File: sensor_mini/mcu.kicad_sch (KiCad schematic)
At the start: 13 parts, among them J2 Programming Header, U8 PIC18LF26K83, U9 MCP2562, Y1 Crystal

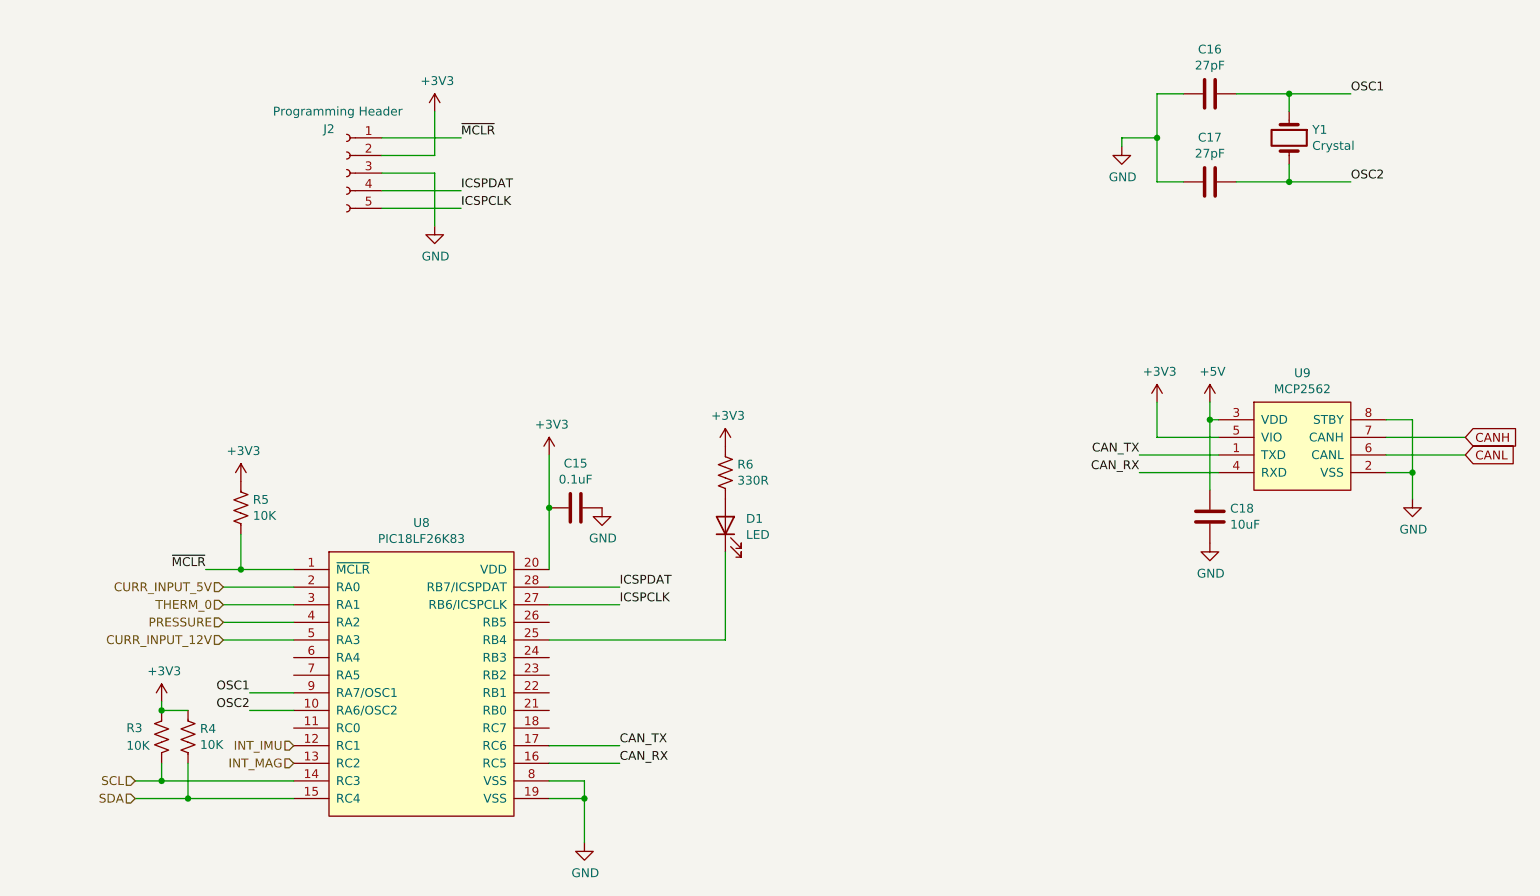
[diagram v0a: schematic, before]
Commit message: Clean Up
Removed old files
Cleaned up Schematics
Created new PDFs
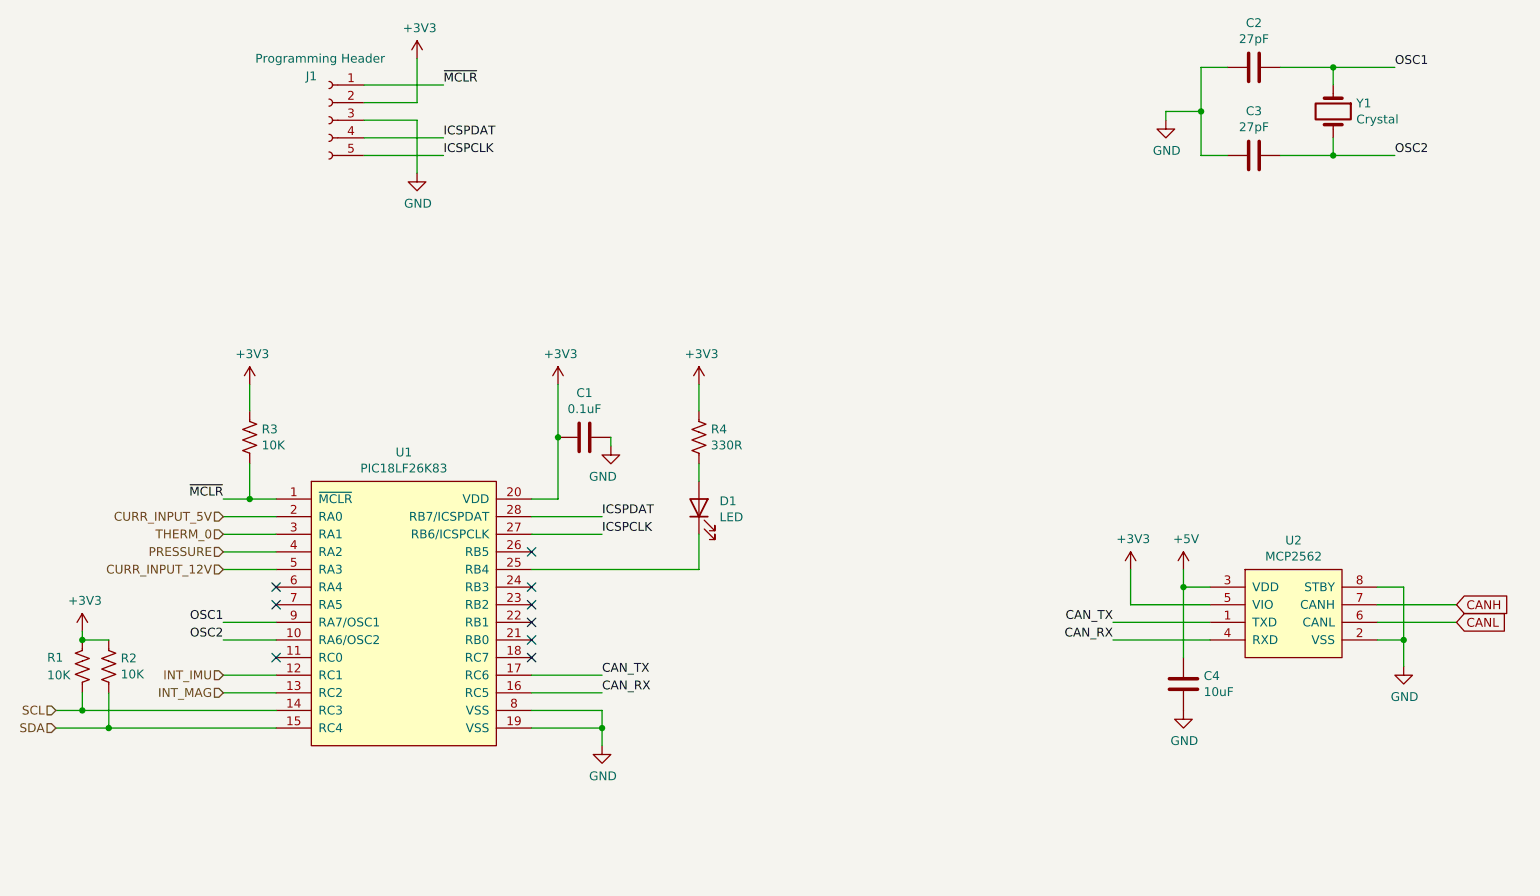
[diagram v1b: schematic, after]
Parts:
- renumbered C15 to C1, C16 to C2, C17 to C3, C18 to C4, J2 to J1, R3 to R1, R4 to R2, R5 to R3, R6 to R4, U8 to U1, U9 to U2
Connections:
- no-connect marks 0 -> 9
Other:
- moved on the sheet: C1, C2, C3, C4, D1, J1, R1, R2, R3, R4, U1, U2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
